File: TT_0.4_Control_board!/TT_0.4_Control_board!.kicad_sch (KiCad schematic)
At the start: 46 parts, among them J1 Conn_01x03_Socket, J10 T4, J11 T5, J12 J_Th, J13 J_Th, J14 J_Th, J15 J_Th, J16 J_BMS_17, J17 J_BMS_23, J18 JST_S_Kill, J2 Pow_Conn, J3 Micro_R, J4 Micro_L, J5 MPU9250, J6 MS5837_30, J7 T1, J8 T2, J9 T3, U1 LM7805_TO220, U2 LM1117T-3.3

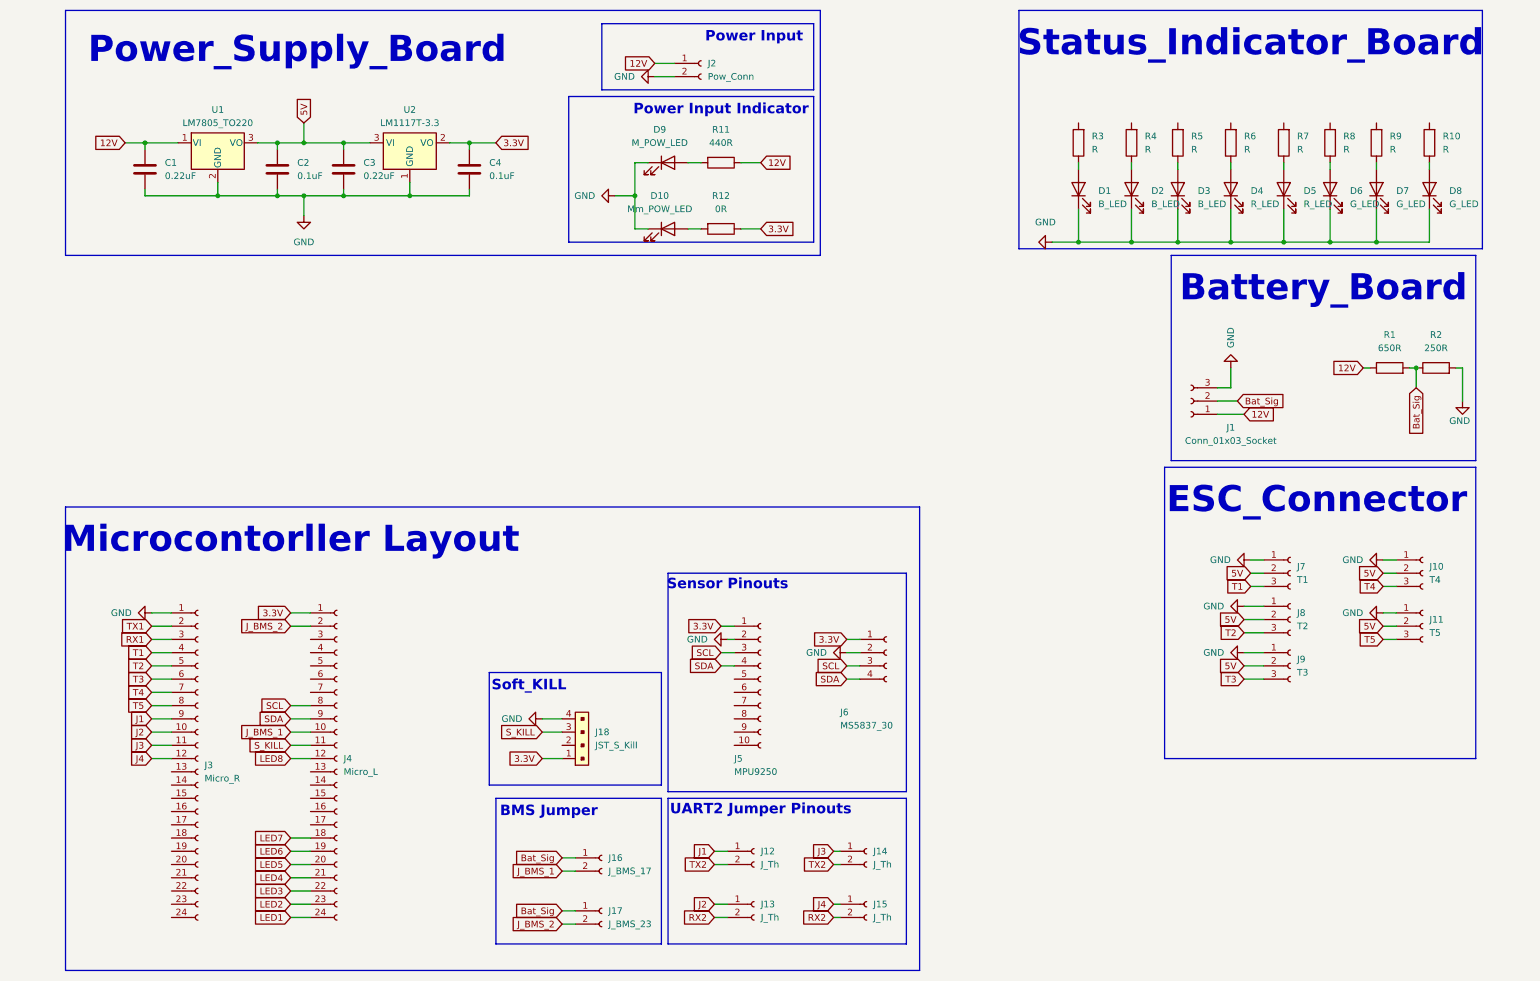
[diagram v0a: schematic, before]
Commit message: Final_PCB_Design
This push final, updated push TT-0.4:Controller
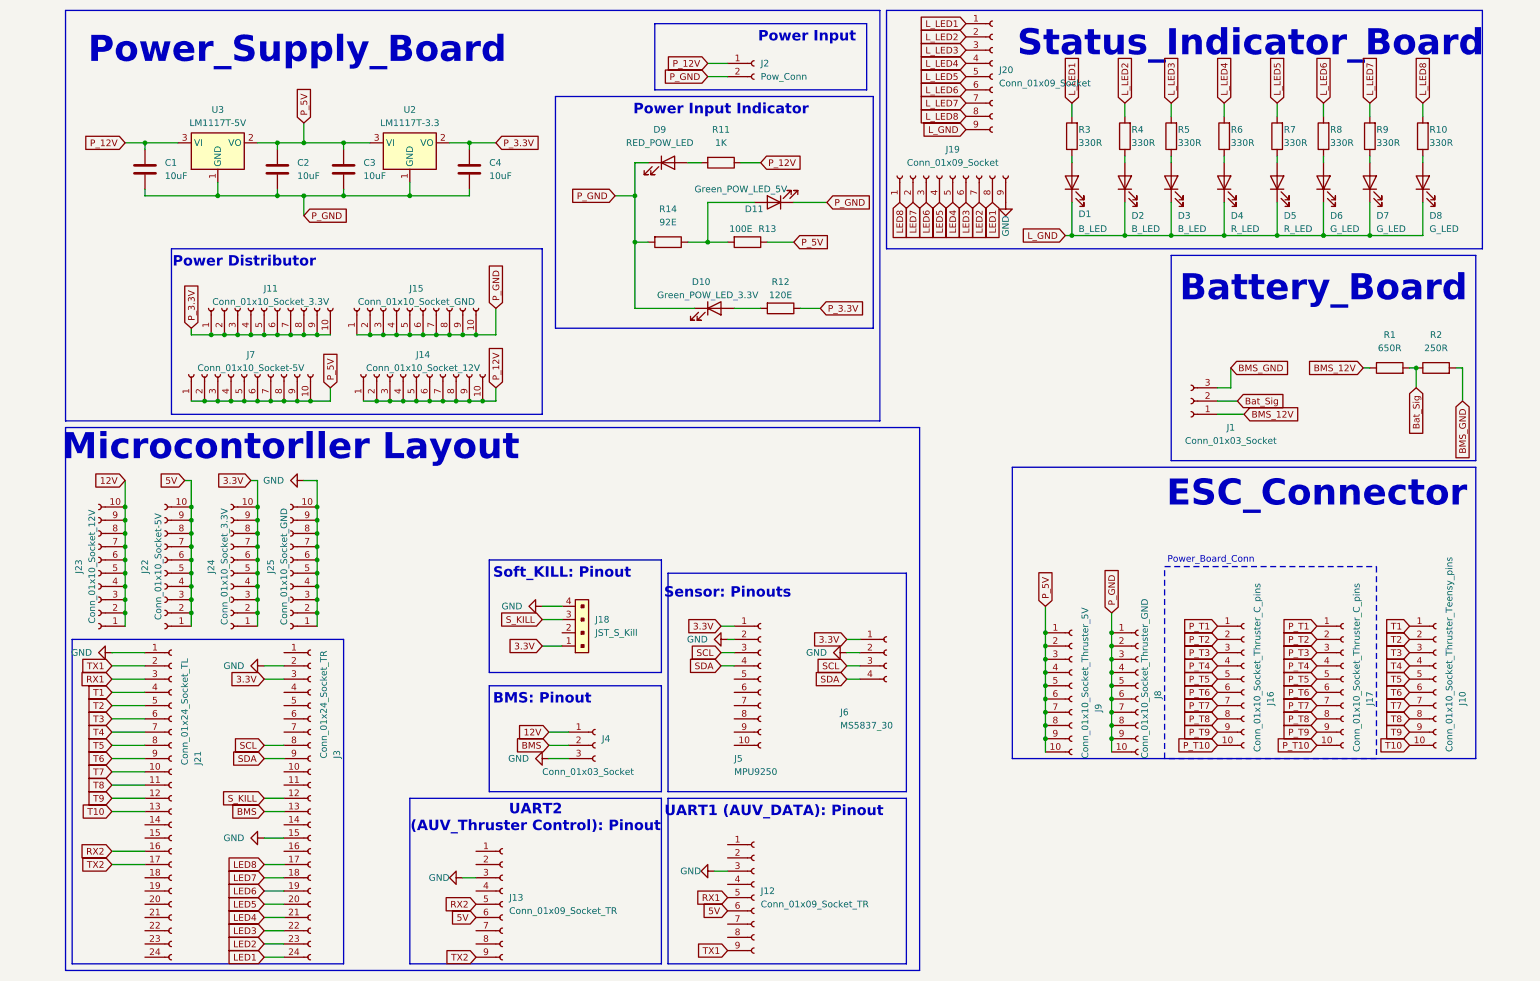
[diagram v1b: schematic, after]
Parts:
- removed J10: T4, symbol Connector:Conn_01x03_Socket
- removed J11: T5, symbol Connector:Conn_01x03_Socket
- removed J12, J13, J14, J15: J_Th, symbol Connector:Conn_01x02_Socket
- removed J16: J_BMS_17, symbol Connector:Conn_01x02_Socket
- removed J17: J_BMS_23, symbol Connector:Conn_01x02_Socket
- removed J4: Micro_L, symbol Connector:Conn_01x24_Socket
- removed J7: T1, symbol Connector:Conn_01x03_Socket
- removed J8: T2, symbol Connector:Conn_01x03_Socket
- removed J9: T3, symbol Connector:Conn_01x03_Socket
- removed U1: LM7805_TO220, Package_TO_SOT_THT:TO-220-3_Vertical, symbol Regulator_Linear:LM7805_TO220
- added D11: Green_POW_LED_5V, LED_THT:LED_D5.0mm, symbol Device:LED
- added J10: Conn_01x10_Socket_Thruster_Teensy_pins, Connector_PinSocket_2.54mm:PinSocket_1x10_P2.54mm_Vertical, symbol Connector:Conn_01x10_Socket
- added J11, J24: Conn_01x10_Socket_3.3V, Connector_PinSocket_2.54mm:PinSocket_1x10_P2.54mm_Vertical, symbol Connector:Conn_01x10_Socket
- added J12, J13: Conn_01x09_Socket_TR, Connector_PinSocket_2.54mm:PinSocket_1x09_P2.54mm_Vertical, symbol Connector:Conn_01x09_Socket
- added J14, J23: Conn_01x10_Socket_12V, Connector_PinSocket_2.54mm:PinSocket_1x10_P2.54mm_Vertical, symbol Connector:Conn_01x10_Socket
- added J15, J25: Conn_01x10_Socket_GND, Connector_PinSocket_2.54mm:PinSocket_1x10_P2.54mm_Vertical, symbol Connector:Conn_01x10_Socket
- added J16, J17: Conn_01x10_Socket_Thruster_C_pins, Connector_PinSocket_2.54mm:PinSocket_1x10_P2.54mm_Vertical, symbol Connector:Conn_01x10_Socket
- added J19, J20: Conn_01x09_Socket, Connector_PinHeader_2.54mm:PinHeader_1x09_P2.54mm_Vertical, symbol Connector:Conn_01x09_Socket
- added J21: Conn_01x24_Socket_TL, Connector_PinSocket_2.54mm:PinSocket_1x24_P2.54mm_Vertical, symbol Connector:Conn_01x24_Socket
- added J22, J7: Conn_01x10_Socket-5V, Connector_PinSocket_2.54mm:PinSocket_1x10_P2.54mm_Vertical, symbol Connector:Conn_01x10_Socket
- added J4: Conn_01x03_Socket, Connector_PinSocket_2.54mm:PinSocket_1x03_P2.54mm_Vertical, symbol Connector:Conn_01x03_Socket
- added J8: Conn_01x10_Socket_Thruster_GND, Connector_PinSocket_2.54mm:PinSocket_1x10_P2.54mm_Vertical, symbol Connector:Conn_01x10_Socket
- added J9: Conn_01x10_Socket_Thruster_5V, Connector_PinSocket_2.54mm:PinSocket_1x10_P2.54mm_Vertical, symbol Connector:Conn_01x10_Socket
- added R13: 100E, Resistor_THT:R_Axial_DIN0207_L6.3mm_D2.5mm_P7.62mm_Horizontal, symbol Device:R
- added R14: 92E, Resistor_THT:R_Axial_DIN0207_L6.3mm_D2.5mm_P7.62mm_Horizontal, symbol Device:R
- added U3: LM1117T-5V, Package_TO_SOT_SMD:SOT-223-3_TabPin2, symbol Regulator_Linear:LM1117T-3.3
- C1, C3: value 0.22uF -> 10uF; footprint (none) -> Capacitor_THT:C_Disc_D7.5mm_W5.0mm_P5.00mm
- C2, C4: value 0.1uF -> 10uF; footprint (none) -> Capacitor_THT:C_Disc_D7.5mm_W5.0mm_P5.00mm
- D1, D2, D3, D4, D5, D6, D7, D8: footprint (none) -> LED_THT:LED_D5.0mm
- D10: value Mm_POW_LED -> Green_POW_LED_3.3V; footprint (none) -> LED_THT:LED_D5.0mm
- D9: value M_POW_LED -> RED_POW_LED; footprint (none) -> LED_THT:LED_D5.0mm
- J1: footprint (none) -> Connector_PinSocket_2.54mm:PinSocket_1x03_P2.54mm_Vertical
- J2: footprint (none) -> TerminalBlock:TerminalBlock_MaiXu_MX126-5.0-02P_1x02_P5.00mm
- J3: value Micro_R -> Conn_01x24_Socket_TR; footprint (none) -> Connector_PinSocket_2.54mm:PinSocket_1x24_P2.54mm_Vertical
- J5: footprint (none) -> Connector_PinSocket_2.54mm:PinSocket_1x10_P2.54mm_Vertical
- J6: footprint (none) -> Connector_PinSocket_2.54mm:PinSocket_1x04_P2.54mm_Vertical
- R1, R2: footprint (none) -> Resistor_THT:R_Axial_DIN0309_L9.0mm_D3.2mm_P15.24mm_Horizontal
- R10, R3, R4, R5, R6, R7, R8, R9: value R -> 330R; footprint (none) -> Resistor_THT:R_Axial_DIN0207_L6.3mm_D2.5mm_P7.62mm_Horizontal
- R11: value 440R -> 1K; footprint (none) -> Resistor_THT:R_Axial_DIN0414_L11.9mm_D4.5mm_P15.24mm_Horizontal
- R12: value 0R -> 120E; footprint (none) -> Resistor_THT:R_Axial_DIN0207_L6.3mm_D2.5mm_P7.62mm_Horizontal
- U2: footprint Package_TO_SOT_THT:TO-220-3_Horizontal_TabDown -> Package_TO_SOT_SMD:SOT-223-3_TabPin2
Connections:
- net J1 is gone; now on net SDA: J3.9 (Pin_9)
- net J4 is gone; now on net S_KILL: J3.12 (Pin_12)
- net 12V: now also J23.1 (Pin_1), J23.10 (Pin_10), J23.2 (Pin_2), J23.3 (Pin_3), J23.4 (Pin_4), J23.5 (Pin_5), J23.6 (Pin_6), J23.7 (Pin_7), J23.8 (Pin_8), J23.9 (Pin_9), J4.1 (Pin_1); no longer C1.1, J1.1 (Pin_1), J2.1 (Pin_1), R1.1, R11.1
- net 3.3V: now also J3.3 (Pin_3), J24.1 (Pin_1), J24.10 (Pin_10), J24.2 (Pin_2), J24.3 (Pin_3), J24.4 (Pin_4), J24.5 (Pin_5), J24.6 (Pin_6), J24.7 (Pin_7), J24.8 (Pin_8), J24.9 (Pin_9); no longer C4.1, R12.1, U2.2 (VO)
- net 5V: now also J12.6 (Pin_6), J13.6 (Pin_6), J22.1 (Pin_1), J22.10 (Pin_10), J22.2 (Pin_2), J22.3 (Pin_3), J22.4 (Pin_4), J22.5 (Pin_5), J22.6 (Pin_6), J22.7 (Pin_7), J22.8 (Pin_8), J22.9 (Pin_9); no longer C2.1, C3.1, U2.3 (VI)
- net GND: now also J3.15 (Pin_15), J3.2 (Pin_2), J12.3 (Pin_3), J13.3 (Pin_3), J19.9 (Pin_9), J21.1 (Pin_1), J25.1 (Pin_1), J25.10 (Pin_10), J25.2 (Pin_2), J25.3 (Pin_3), J25.4 (Pin_4), J25.5 (Pin_5), J25.6 (Pin_6), J25.7 (Pin_7), J25.8 (Pin_8), J25.9 (Pin_9), J4.3 (Pin_3); no longer C1.2, C2.2, C3.2, C4.2, D1.1 (K), D10.1 (K), D2.1 (K), D3.1 (K), D4.1 (K), D5.1 (K), D6.1 (K), D7.1 (K), D8.1 (K), D9.1 (K), J1.3 (Pin_3), J2.2 (Pin_2), J3.1 (Pin_1), R2.2, U2.1 (GND)
- net LED1: now also J3.24 (Pin_24), J19.8 (Pin_8)
- net LED2: now also J3.23 (Pin_23), J19.7 (Pin_7)
- net LED3: now also J3.22 (Pin_22), J19.6 (Pin_6)
- net LED4: now also J3.21 (Pin_21), J19.5 (Pin_5)
- net LED5: now also J3.20 (Pin_20), J19.4 (Pin_4)
- net LED6: now also J3.19 (Pin_19), J19.3 (Pin_3)
- net LED7: now also J3.18 (Pin_18), J19.2 (Pin_2)
- net LED8: now also J3.17 (Pin_17), J19.1 (Pin_1)
- net RX1: now also J12.5 (Pin_5), J21.3 (Pin_3); no longer J3.3 (Pin_3)
- net RX2: now also J13.5 (Pin_5), J21.16 (Pin_16)
- net SCL: now also J3.8 (Pin_8)
- net T1: now also J10.1 (Pin_1), J21.4 (Pin_4); no longer J3.4 (Pin_4)
- net T2: now also J10.2 (Pin_2), J21.5 (Pin_5); no longer J3.5 (Pin_5)
- net T3: now also J10.3 (Pin_3), J21.6 (Pin_6); no longer J3.6 (Pin_6)
- net T4: now also J10.4 (Pin_4), J21.7 (Pin_7); no longer J3.7 (Pin_7)
- net T5: now also J10.5 (Pin_5), J21.8 (Pin_8); no longer J3.8 (Pin_8)
- net TX1: now also J12.9 (Pin_9), J21.2 (Pin_2); no longer J3.2 (Pin_2)
- net TX2: now also J13.9 (Pin_9), J21.17 (Pin_17)
- net L_LED7: now reaches R9.2
- net L_LED7: now also J20.7 (Pin_7)
- net L_LED2: now reaches R4.2
- net L_LED2: now also J20.2 (Pin_2)
- net L_LED3: now reaches R5.2
- net L_LED3: now also J20.3 (Pin_3)
- net L_LED1: now reaches R3.2
- net L_LED1: now also J20.1 (Pin_1)
- net L_LED5: now reaches R7.2
- net L_LED5: now also J20.5 (Pin_5)
- net L_LED4: now reaches R6.2
- net L_LED4: now also J20.4 (Pin_4)
- net BMS: now reaches J3.13 (Pin_13)
- net BMS: now also J4.2 (Pin_2)
- net L_LED8: now reaches R10.2
- net L_LED8: now also J20.8 (Pin_8)
- net L_LED6: now reaches R8.2
- net L_LED6: now also J20.6 (Pin_6)
- net J2: no longer names the net of J3.10 (Pin_10)
- net J3: no longer names the net of J3.11 (Pin_11)
- new net: D11.2 (A), R13.2, R14.1
- new net BMS_12V: J1.1 (Pin_1), R1.1
- new net BMS_GND: J1.3 (Pin_3), R2.2
- new net L_GND: D1.1 (K), D2.1 (K), D3.1 (K), D4.1 (K), D5.1 (K), D6.1 (K), D7.1 (K), D8.1 (K), J20.9 (Pin_9)
- new net P_12V: C1.1, J14.1 (Pin_1), J14.10 (Pin_10), J14.2 (Pin_2), J14.3 (Pin_3), J14.4 (Pin_4), J14.5 (Pin_5), J14.6 (Pin_6), J14.7 (Pin_7), J14.8 (Pin_8), J14.9 (Pin_9), J2.1 (Pin_1), R11.1, U3.3 (VI)
- new net P_3.3V: C4.1, J11.1 (Pin_1), J11.10 (Pin_10), J11.2 (Pin_2), J11.3 (Pin_3), J11.4 (Pin_4), J11.5 (Pin_5), J11.6 (Pin_6), J11.7 (Pin_7), J11.8 (Pin_8), J11.9 (Pin_9), R12.1, U2.2 (VO)
- new net P_5V: C2.1, C3.1, J7.1 (Pin_1), J7.10 (Pin_10), J7.2 (Pin_2), J7.3 (Pin_3), J7.4 (Pin_4), J7.5 (Pin_5), J7.6 (Pin_6), J7.7 (Pin_7), J7.8 (Pin_8), J7.9 (Pin_9), J9.1 (Pin_1), J9.10 (Pin_10), J9.2 (Pin_2), J9.3 (Pin_3), J9.4 (Pin_4), J9.5 (Pin_5), J9.6 (Pin_6), J9.7 (Pin_7), J9.8 (Pin_8), J9.9 (Pin_9), R13.1, U2.3 (VI), U3.2 (VO)
- new net P_GND: C1.2, C2.2, C3.2, C4.2, D10.1 (K), D11.1 (K), D9.1 (K), J15.1 (Pin_1), J15.10 (Pin_10), J15.2 (Pin_2), J15.3 (Pin_3), J15.4 (Pin_4), J15.5 (Pin_5), J15.6 (Pin_6), J15.7 (Pin_7), J15.8 (Pin_8), J15.9 (Pin_9), J2.2 (Pin_2), J8.1 (Pin_1), J8.10 (Pin_10), J8.2 (Pin_2), J8.3 (Pin_3), J8.4 (Pin_4), J8.5 (Pin_5), J8.6 (Pin_6), J8.7 (Pin_7), J8.8 (Pin_8), J8.9 (Pin_9), R14.2, U2.1 (GND), U3.1 (GND)
- new net P_T1: J16.1 (Pin_1), J17.1 (Pin_1)
- new net P_T10: J16.10 (Pin_10), J17.10 (Pin_10)
- new net P_T2: J16.2 (Pin_2), J17.2 (Pin_2)
- new net P_T3: J16.3 (Pin_3), J17.3 (Pin_3)
- new net P_T4: J16.4 (Pin_4), J17.4 (Pin_4)
- new net P_T5: J16.5 (Pin_5), J17.5 (Pin_5)
- new net P_T6: J16.6 (Pin_6), J17.6 (Pin_6)
- new net P_T7: J16.7 (Pin_7), J17.7 (Pin_7)
- new net P_T8: J16.8 (Pin_8), J17.8 (Pin_8)
- new net P_T9: J16.9 (Pin_9), J17.9 (Pin_9)
- new net T10: J10.10 (Pin_10), J21.13 (Pin_13)
- new net T6: J10.6 (Pin_6), J21.9 (Pin_9)
- new net T7: J10.7 (Pin_7), J21.10 (Pin_10)
- new net T8: J10.8 (Pin_8), J21.11 (Pin_11)
- new net T9: J10.9 (Pin_9), J21.12 (Pin_12)
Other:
- note added: "BMS: Pinout"
- note added: "Power Distributor"
- note added: "Power_Board_Conn"
- note added: "Sensor: Pinouts"
- note added: "Soft_KILL: Pinout"
- note added: "UART1 (AUV_DATA): Pinout"
- note added: "UART2 (AUV_Thruster Control): Pinout"
- note removed: "BMS Jumper"
- note removed: "Sensor Pinouts"
- note removed: "Soft_KILL"
- note removed: "UART2 Jumper Pinouts"
- moved on the sheet: D1, D10, D2, D3, D4, D5, D6, D7, D8, J18, J2, R10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
